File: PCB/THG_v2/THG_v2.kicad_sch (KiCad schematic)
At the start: 11 parts, among them J1 AM2315_Jack, J2 LCD_conn, J3 RTC_Conn, J4 SD_card_conn, J5 AC_in_terminal, U1 mini_esp32

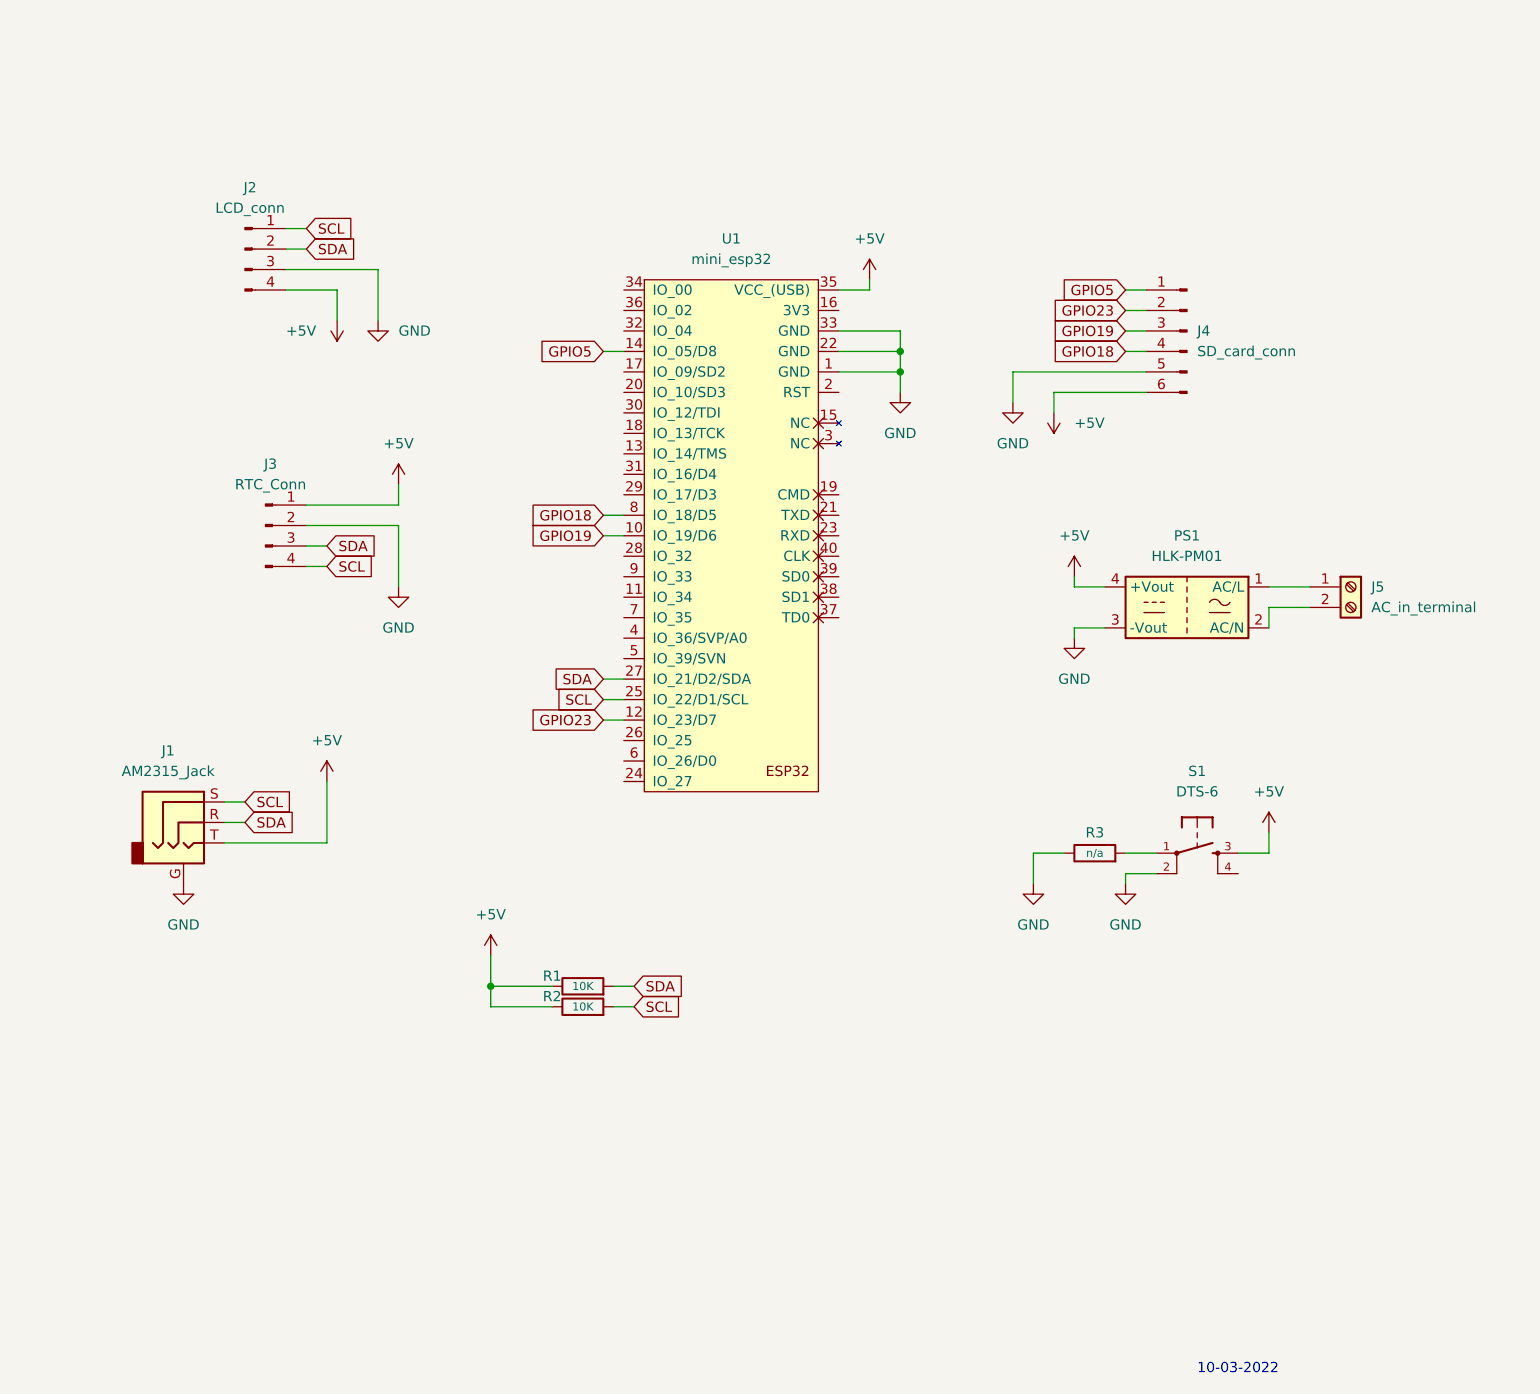
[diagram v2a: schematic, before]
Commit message: revisi
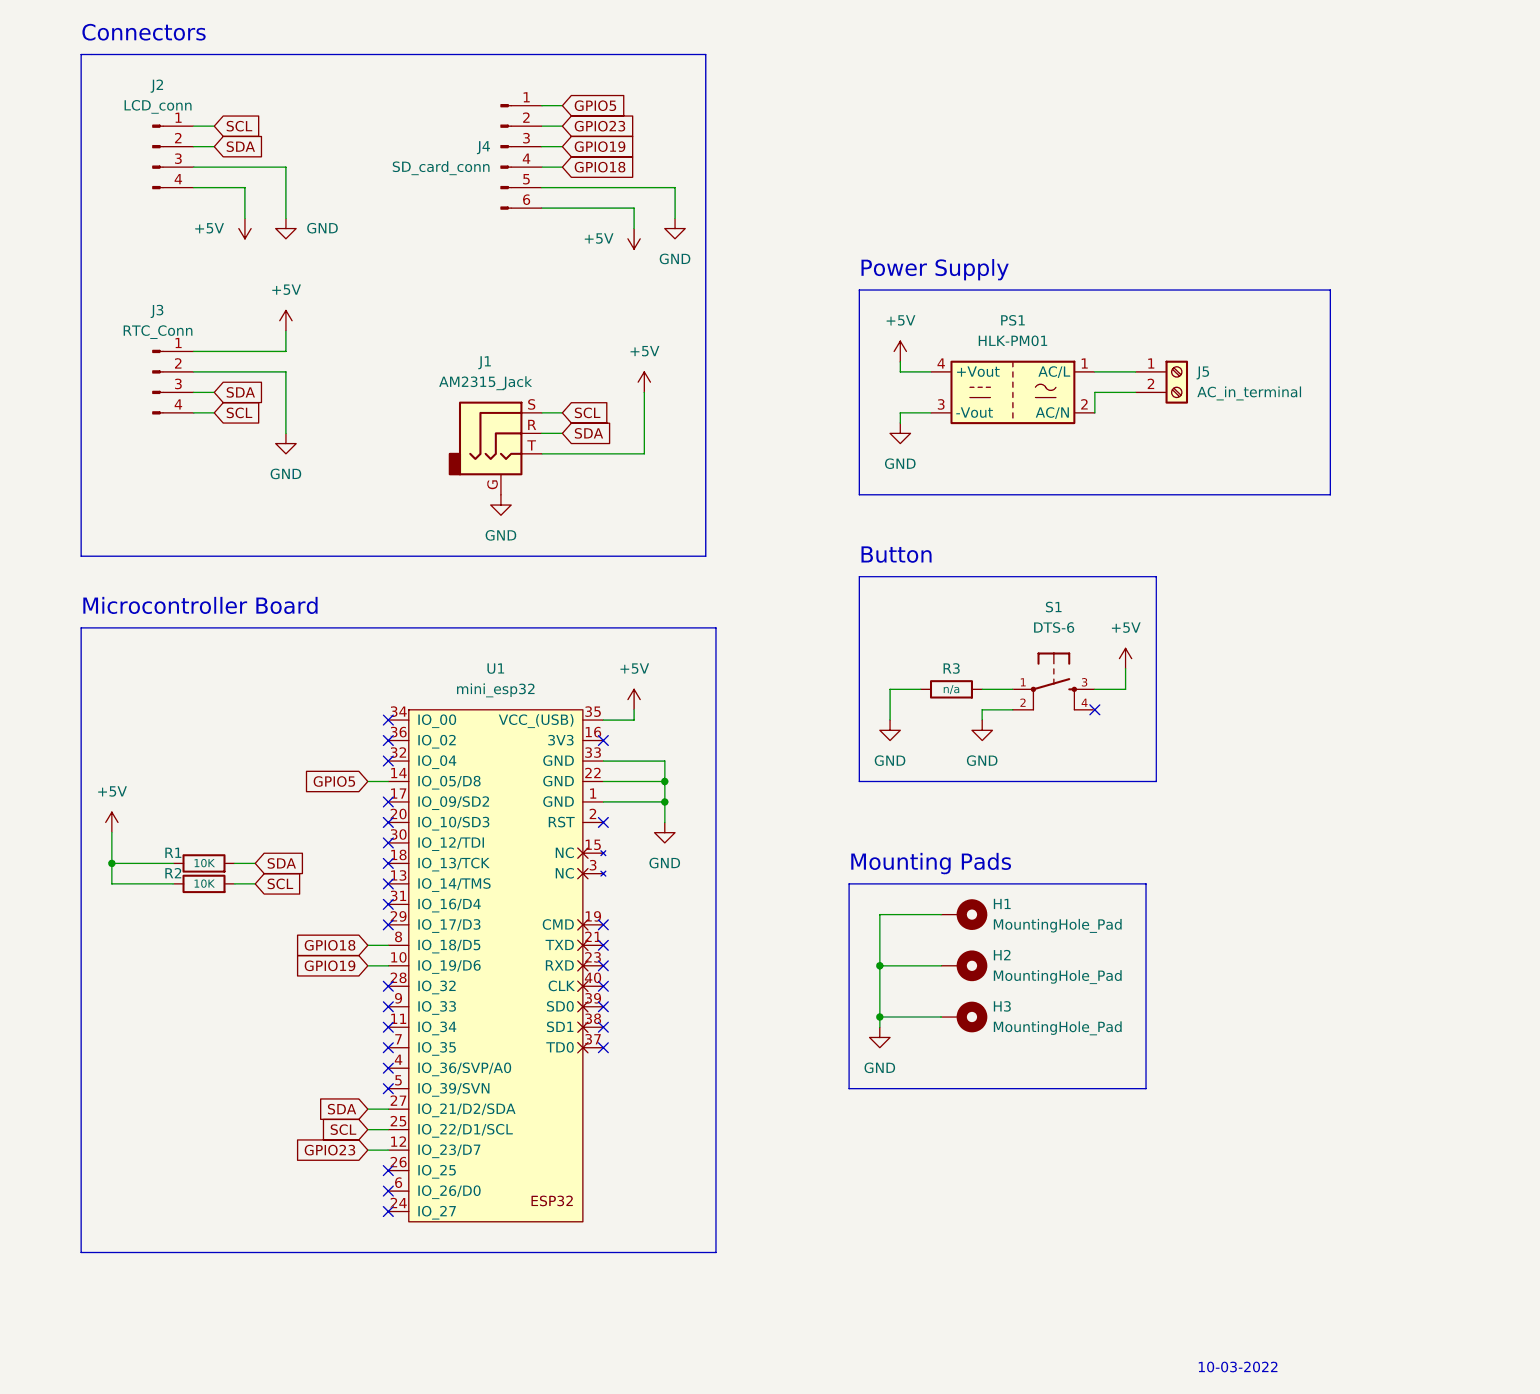
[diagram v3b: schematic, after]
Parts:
- added H1, H2, H3: MountingHole_Pad, MountingHole:MountingHole_2.2mm_M2_Pad_Via, symbol Mechanical:MountingHole_Pad
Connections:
- net GND: now also H1.1, H2.1, H3.1
- no-connect marks 0 -> 29
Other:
- note added: "Button"
- note added: "Connectors"
- note added: "Microcontroller Board"
- note added: "Mounting Pads"
- note added: "Power Supply"
- moved on the sheet: J1, J2, J3, J4, J5, PS1, R1, R2, R3, S1, U1
